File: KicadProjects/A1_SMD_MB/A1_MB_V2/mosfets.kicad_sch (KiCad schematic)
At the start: 24 parts, among them J6 THB2, J7 HE, J8 HE, J9 THB1, Q1 NMOS, Q2 NMOS

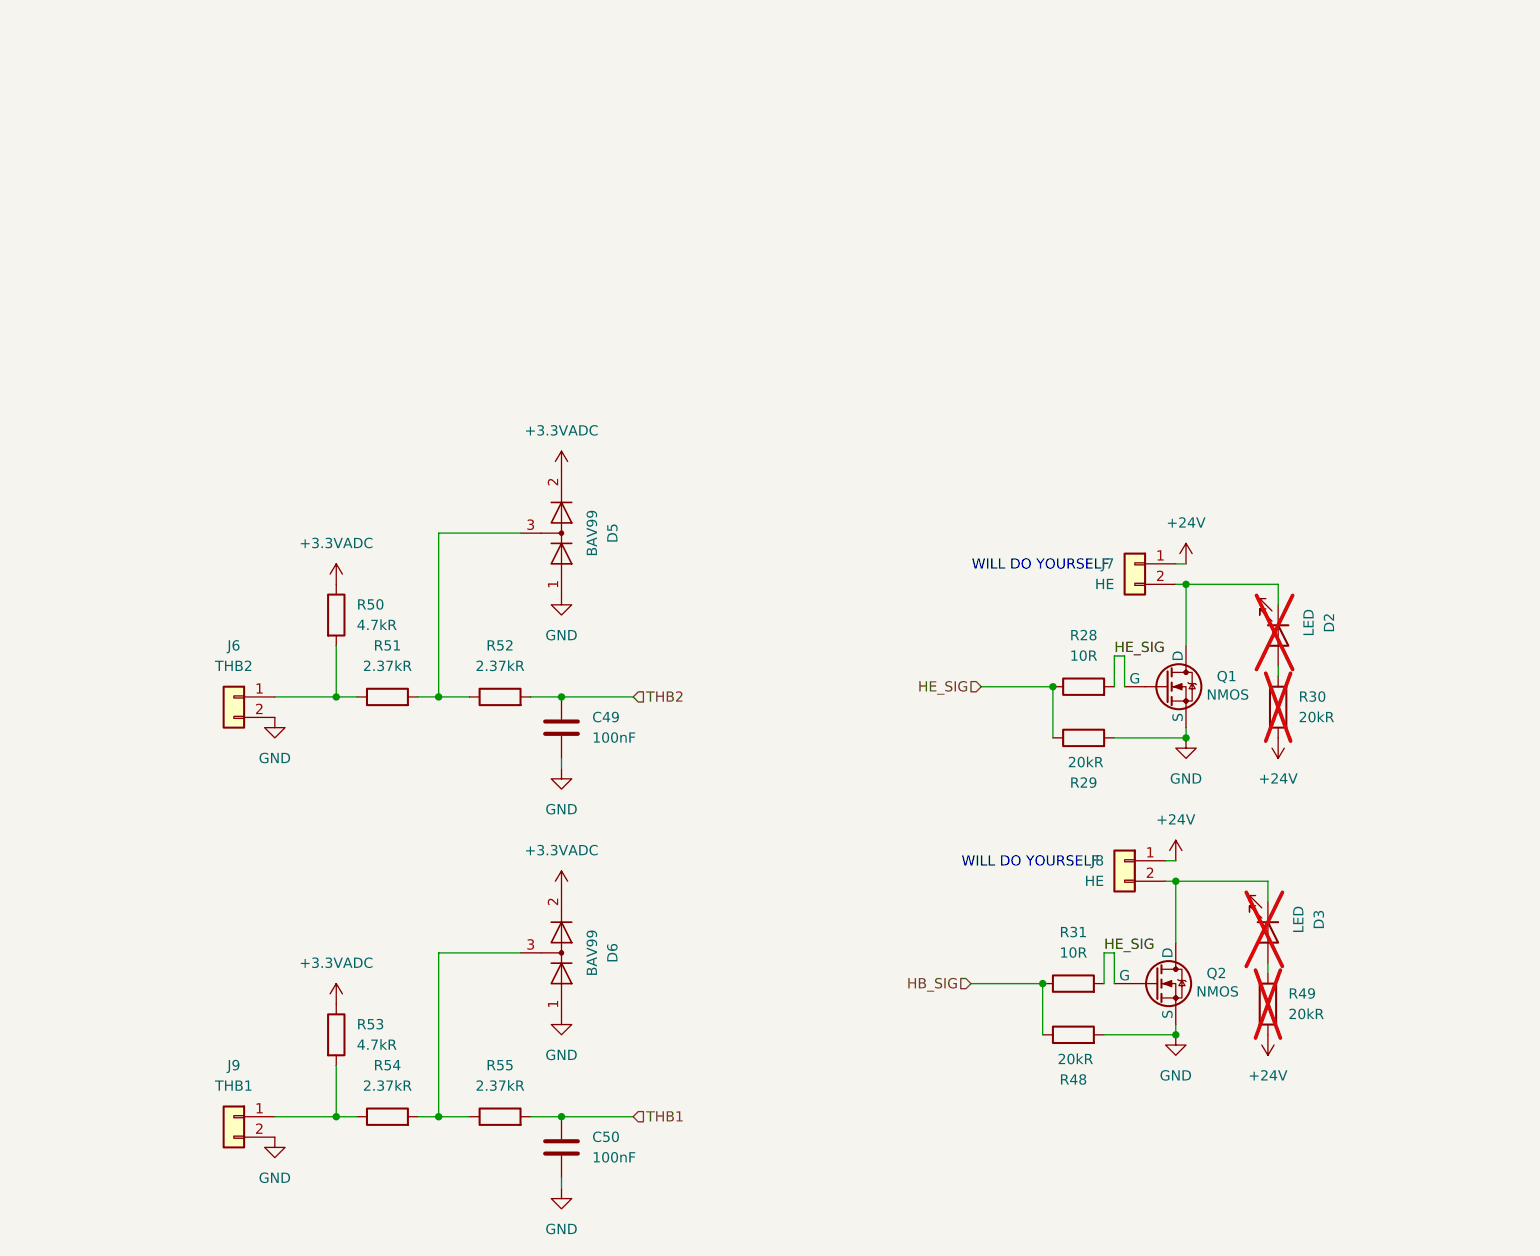
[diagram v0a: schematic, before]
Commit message: e
e
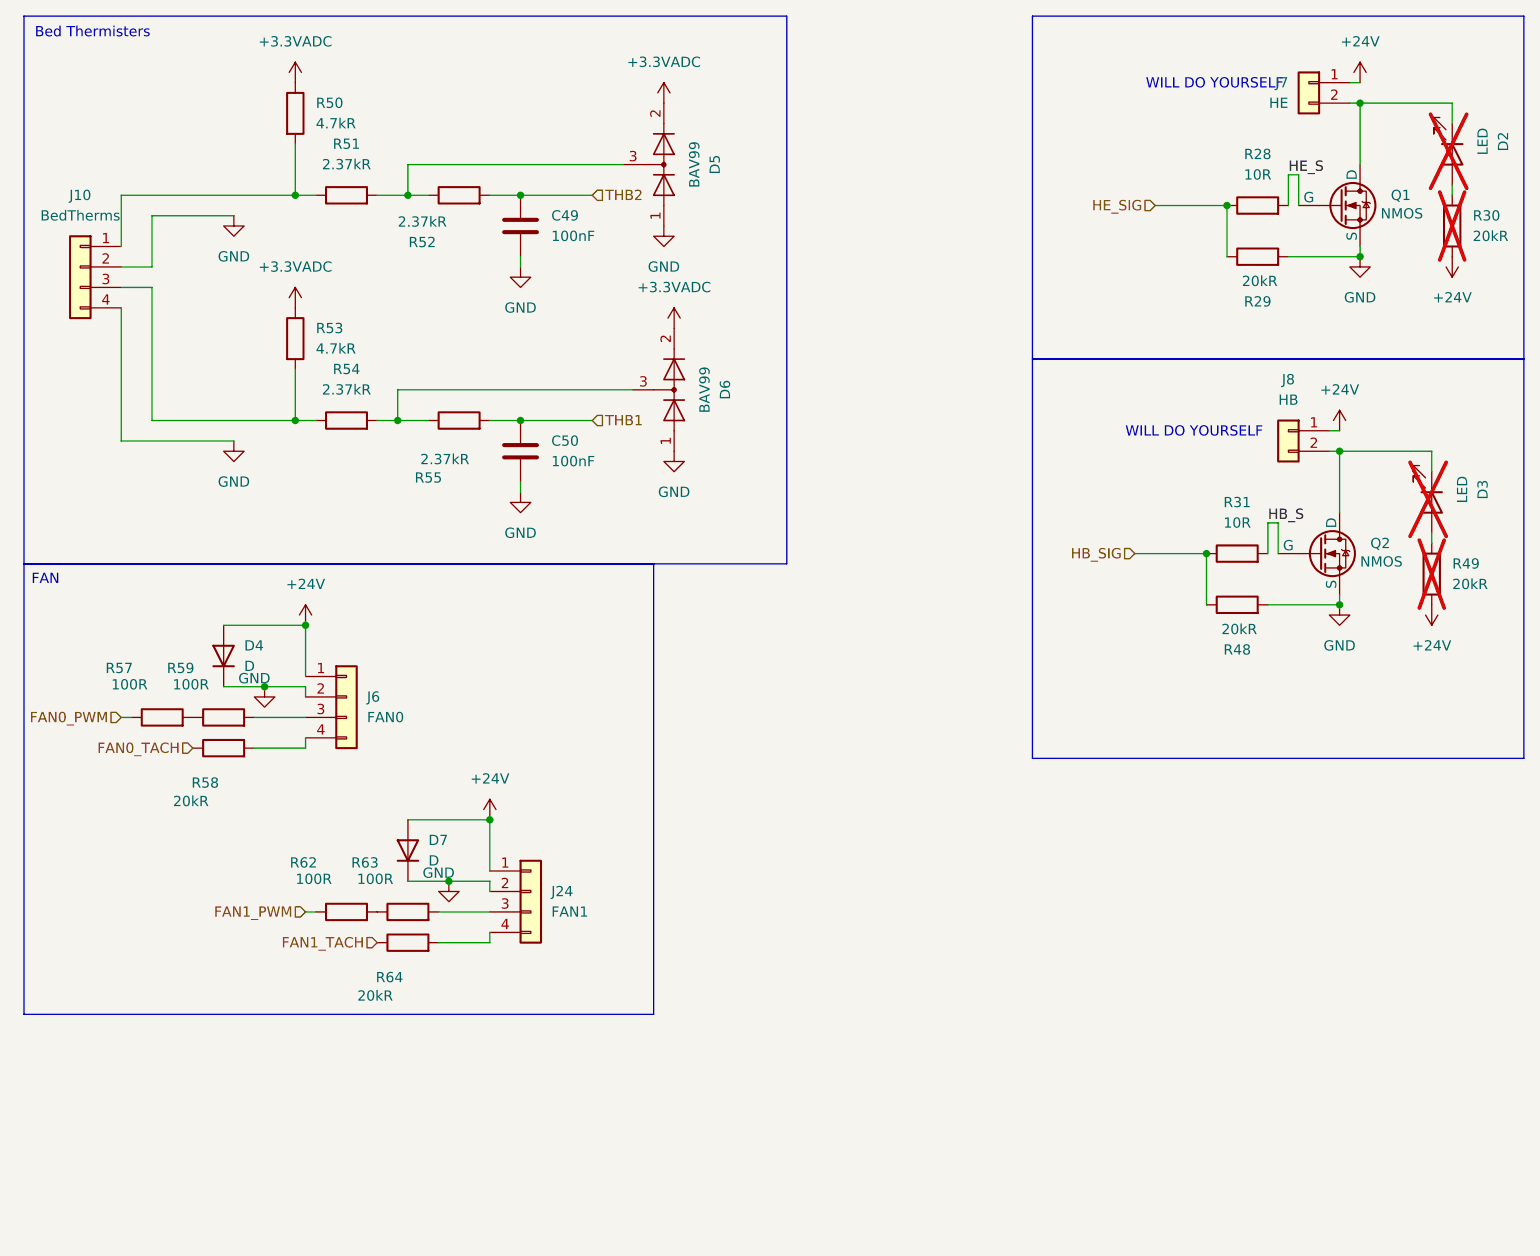
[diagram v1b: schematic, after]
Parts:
- removed J6: THB2, Connector_JST:JST_XH_B2B-XH-A_1x02_P2.50mm_Vertical, symbol Connector_Generic:Conn_01x02
- removed J9: THB1, Connector_JST:JST_XH_B2B-XH-A_1x02_P2.50mm_Vertical, symbol Connector_Generic:Conn_01x02
- added D4, D7: D, Diode_SMD:D_SMA, symbol Device:D
- added J10: BedTherms, Connector_JST:JST_XH_B4B-XH-A_1x04_P2.50mm_Vertical, symbol Connector_Generic:Conn_01x04
- added J24: FAN1, Connector_JST:JST_XH_B4B-XH-A_1x04_P2.50mm_Vertical, symbol Connector_Generic:Conn_01x04
- added J6: FAN0, Connector_JST:JST_XH_B4B-XH-A_1x04_P2.50mm_Vertical, symbol Connector_Generic:Conn_01x04
- added R57, R59, R62, R63: 100R, Resistor_SMD:R_0402_1005Metric, symbol Device:R
- added R58, R64: 20kR, Resistor_SMD:R_0402_1005Metric, symbol Device:R
- J7: footprint Connector_JST:JST_XH_B2B-XH-A_1x02_P2.50mm_Vertical -> OpenA1K:ScrewTerminal 7mm x 7mm
- J8: value HE -> HB; footprint Connector_JST:JST_XH_B2B-XH-A_1x02_P2.50mm_Vertical -> OpenA1K:ScrewTerminal 7mm x 7mm
- Q1, Q2: footprint A1_SMD_THB:sot23f -> Package_TO_SOT_SMD:SOT-23-3
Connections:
- net +24V: now also D4.2 (A), D7.2 (A), J24.1 (Pin_1), J6.1 (Pin_1)
- net GND: now also D4.1 (K), D7.1 (K), J10.2 (Pin_2), J10.4 (Pin_4), J24.2 (Pin_2), J6.2 (Pin_2)
- net HE_SIG: no longer Q1.2 (G), Q2.2 (G), R28.2, R31.2
- net at R50.2, R51.1: now also J10.1 (Pin_1)
- net at R53.2, R54.1: now also J10.3 (Pin_3)
- new net: J6.4 (Pin_4), R58.2
- new net: J24.3 (Pin_3), R63.2
- new net: J24.4 (Pin_4), R64.2
- new net: R62.2, R63.1
- new net: J6.3 (Pin_3), R59.2
- new net: R57.2, R59.1
- new net FAN0_PWM: R57.1
- new net FAN0_TACH: R58.1
- new net FAN1_PWM: R62.1
- new net FAN1_TACH: R64.1
- new net HB_S: Q2.2 (G), R31.2
- new net HE_S: Q1.2 (G), R28.2
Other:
- note added: "Bed Thermisters"
- note added: "FAN"
- moved on the sheet: C49, C50, D2, D3, D5, D6, J7, J8, Q1, Q2, R28, R29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
